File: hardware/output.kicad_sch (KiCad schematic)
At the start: 12 parts

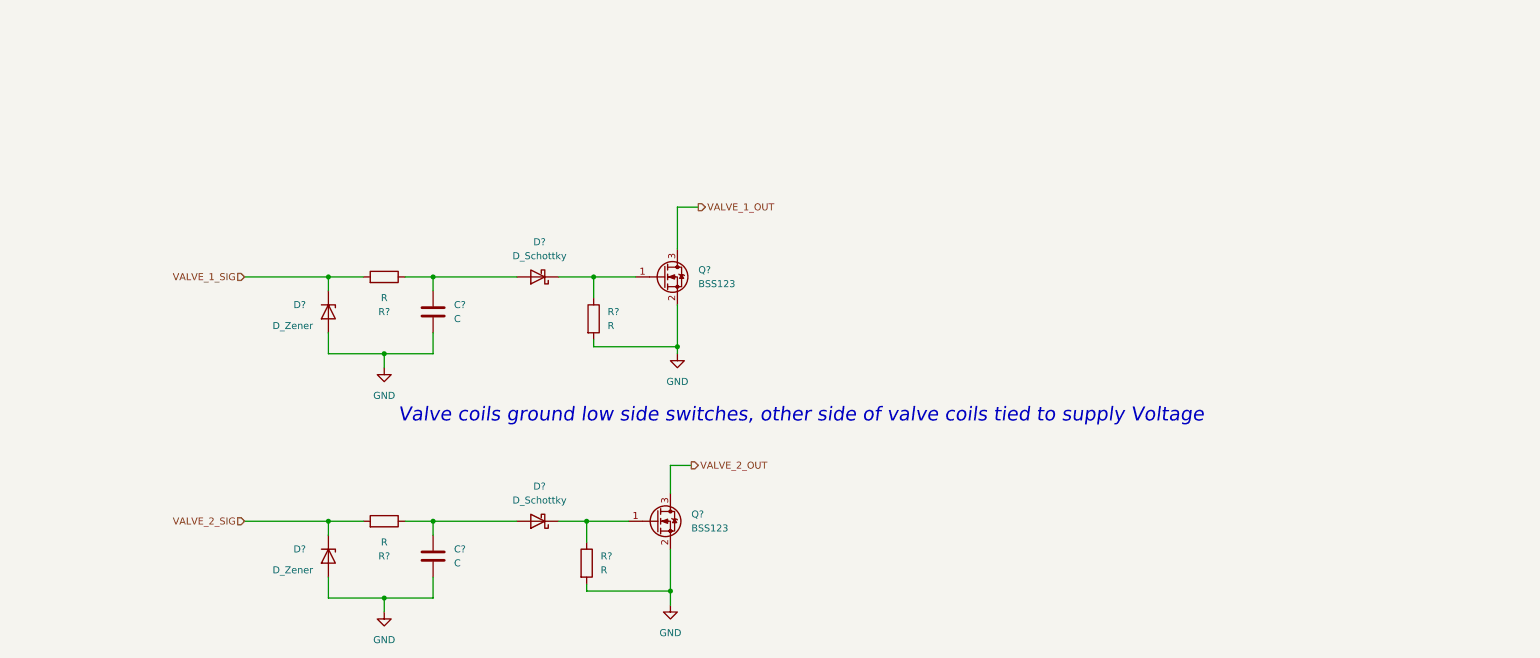
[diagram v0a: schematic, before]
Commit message: Fixed Logic
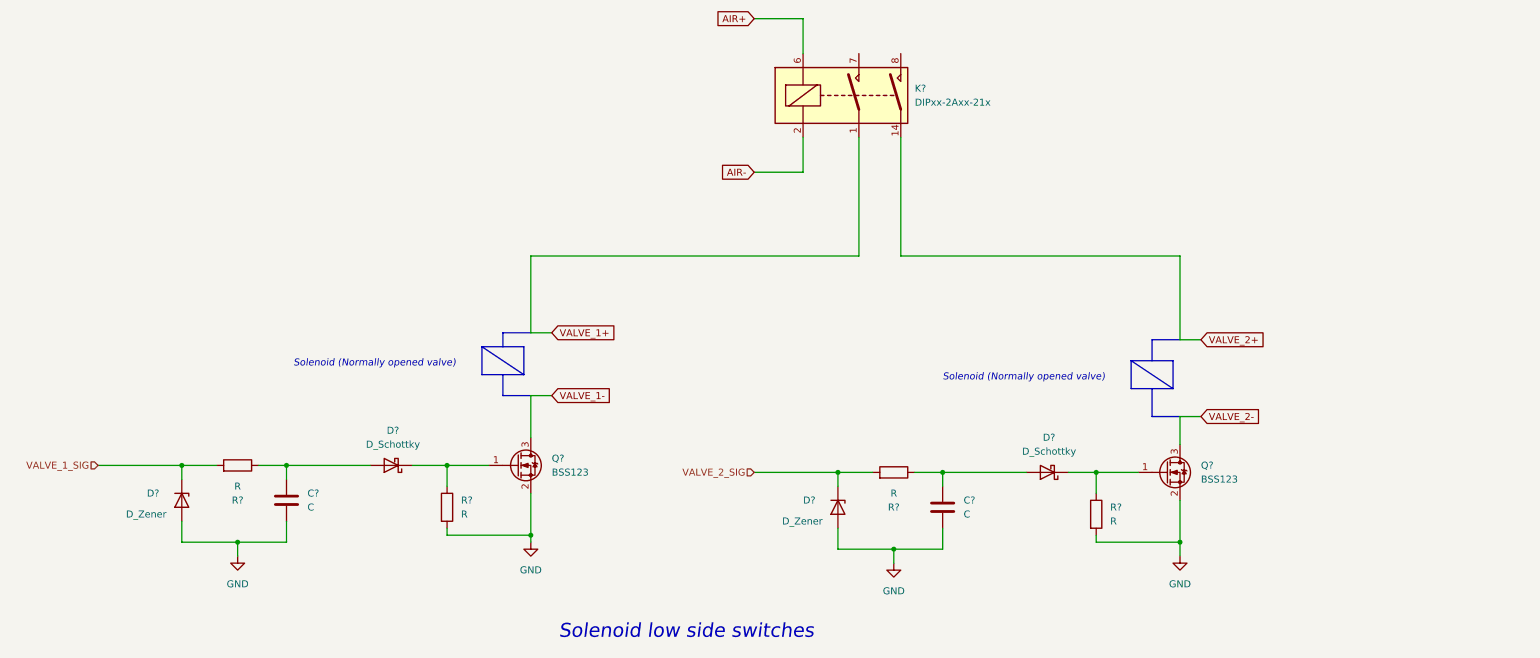
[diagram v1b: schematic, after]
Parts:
- added K?: DIPxx-2Axx-21x, Relay_THT:Relay_StandexMeder_DIP_LowProfile, symbol Relay:DIPxx-2Axx-21x
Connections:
- net VALVE_1_OUT renamed VALVE_1-
- net VALVE_2_OUT renamed VALVE_2-
- new net AIR+: K?.6
- new net AIR-: K?.2
- new net VALVE_1+: K?.1
- new net VALVE_2+: K?.14
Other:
- note added: "Solenoid (Normally opened valve)"
- note added: "Solenoid low side switches"
- note removed: "Valve coils ground low side switches, other side of valve coils tied to supply Voltage"
- moved on the sheet: C?, D?, Q?, R?
